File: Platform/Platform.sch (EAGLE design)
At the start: 30 parts, among them U1 LCD-16X2NOSILK, U2 LM2574N, X1 USBSMD, Y1 RESONATORSMD

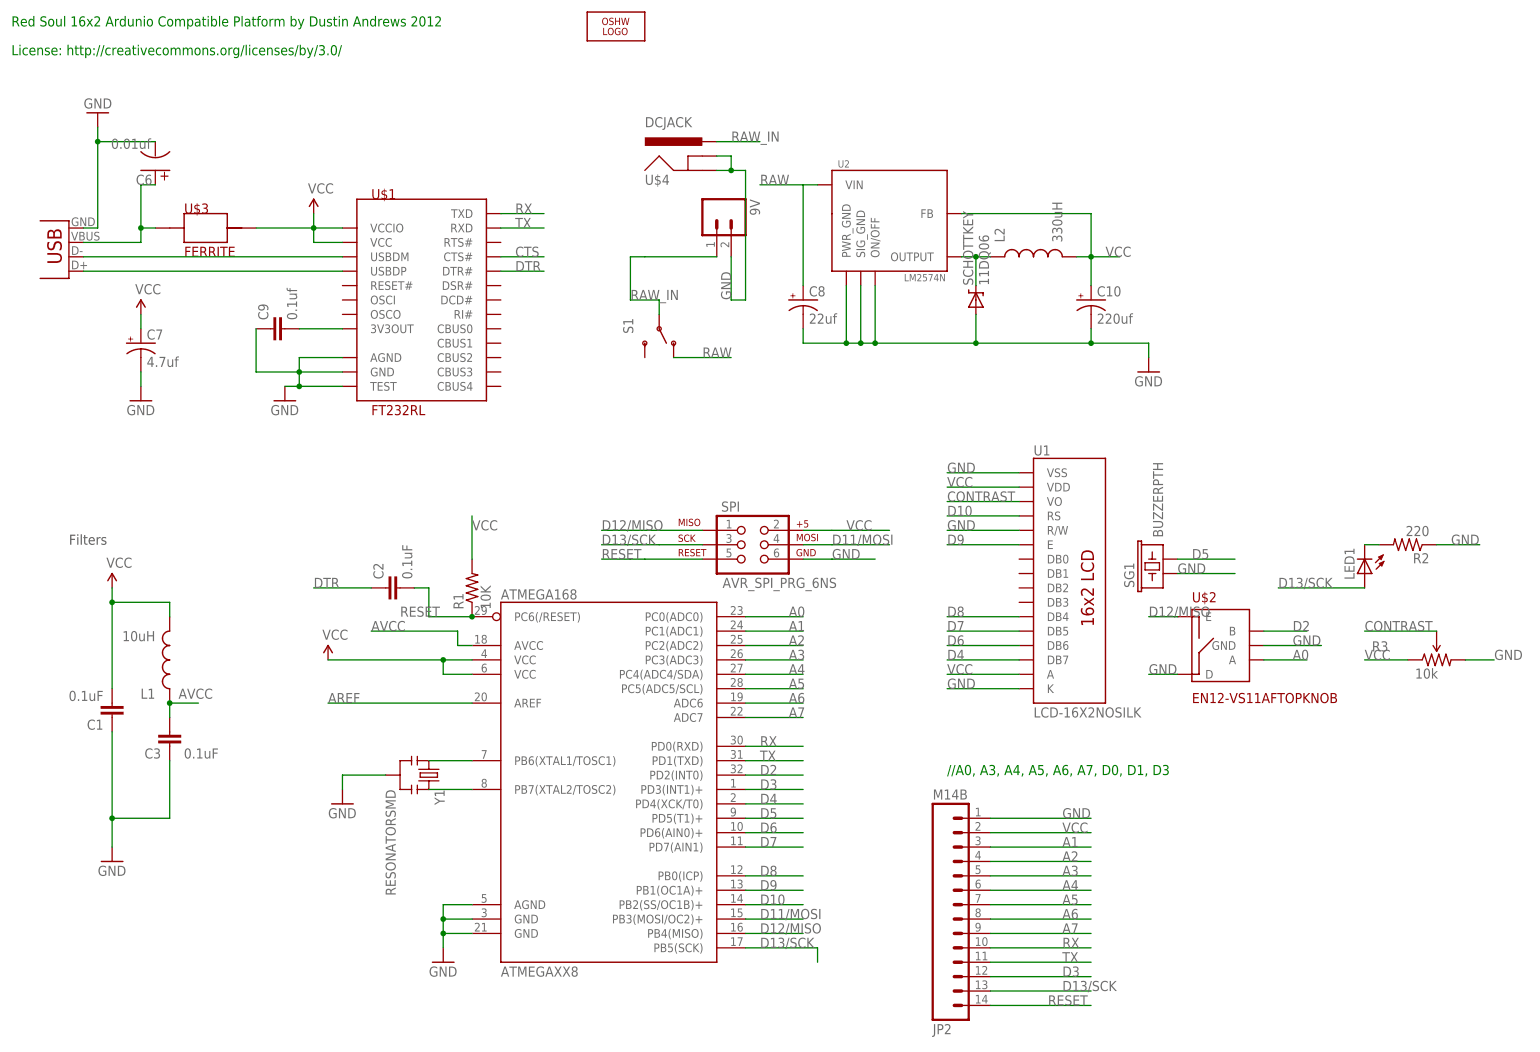
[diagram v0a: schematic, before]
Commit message: prototype 3
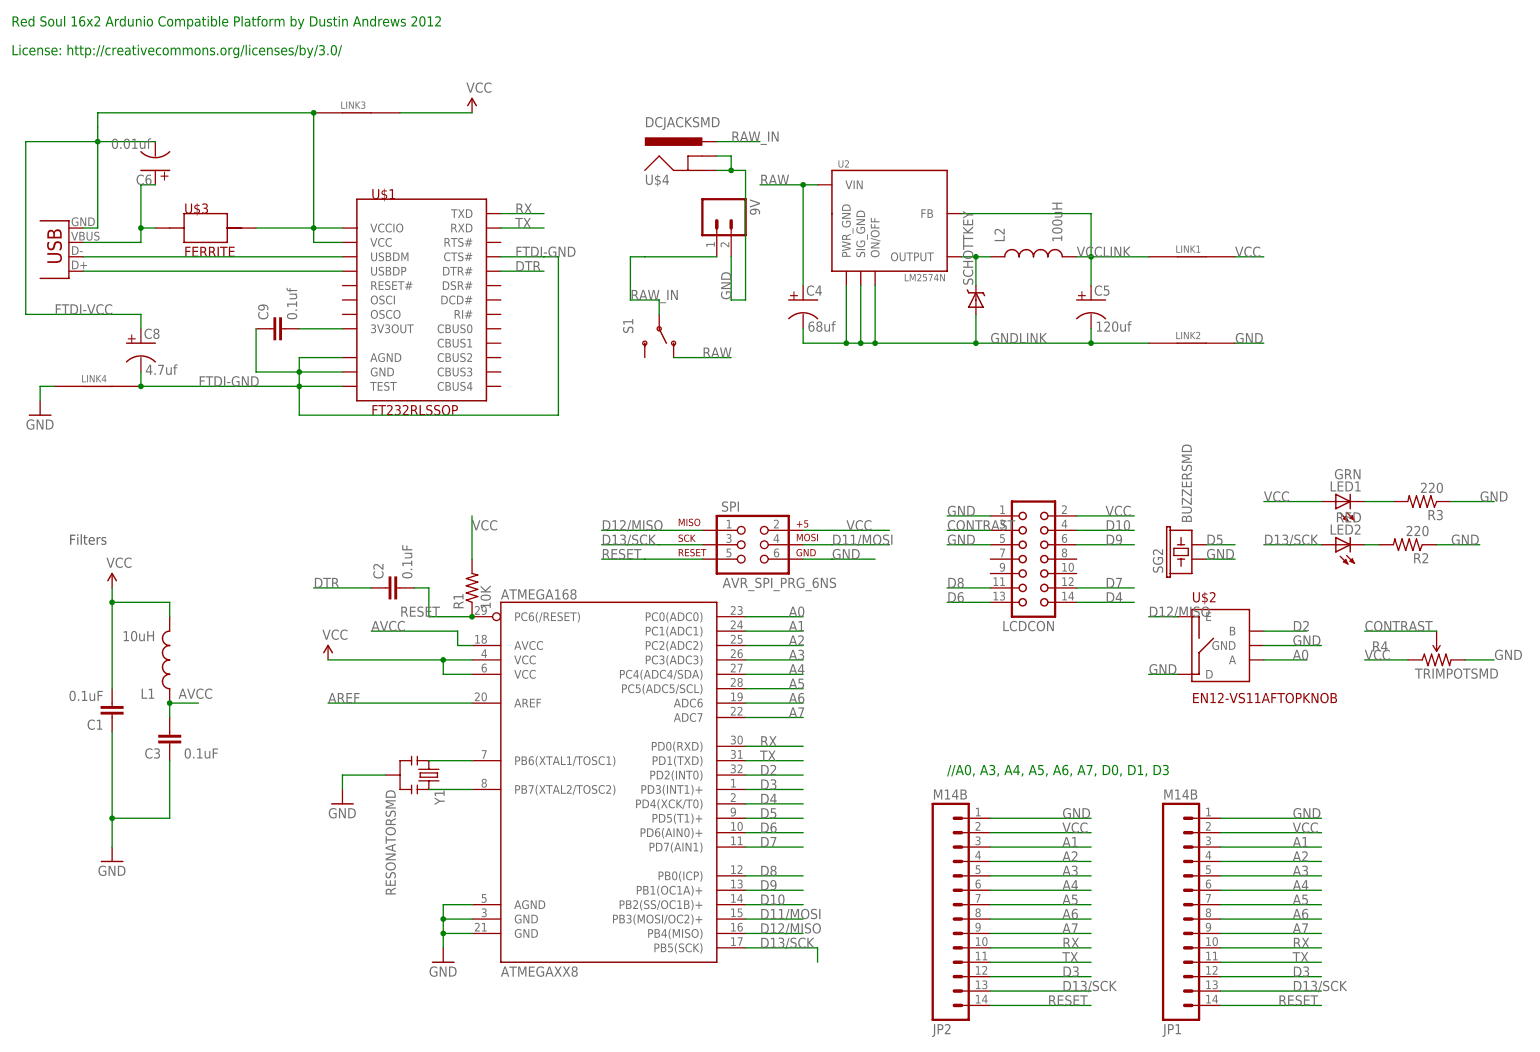
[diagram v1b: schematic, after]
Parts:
- removed C10: 220uf, SparkFun:CAP_POLPTH1
- removed C7: 4.7uf, SparkFun:CAP_POLPTH1
- removed LOGO1: OSHW_LOGO_10MIL, ohw-logo:OSHW_LOGO_10MIL
- removed SG1: BUZZERPTH, SparkFun:BUZZERPTH
- removed U1: LCD-16X2NOSILK, SparkFun:LCD-16X2NOSILK
- added C4: 68uf, Dustin:CAP_POLF80
- added C5: 120uf, Dustin:CAP_POL8X10
- added JP1: M14B, Dustin:M14B
- added LCDCON: (no value), con-harting:CON14
- added LED2: RED, SparkFun:LED1206
- added LINK1, LINK2, LINK3, LINK4: LINK, Dustin:LINK
- added R4: TRIMPOTSMD, SparkFun:TRIMPOTSMD
- added SG2: BUZZERSMD, SparkFun:BUZZERSMD
- C8: value 22uf -> 4.7uf; device SparkFun:CAP_POLPTH1 -> Dustin:CAP_POLCAP-B
- L2: value 330uH -> 100uH; device SparkFun:INDUCTOR1206H* -> SparkFun:INDUCTOR0805
- LED1: value (none) -> GRN; device SparkFun:LED3MM -> SparkFun:LED1206
- R3: value 10k -> 220; device SparkFun:TRIMPOTPTH -> SparkFun:RESISTOR0805-RES
- SCHOTTKEY: value 11DQ06 -> DIODE-SCHOTTKY; device SparkFun:DIODE-ZENERPTH -> Dustin:DIODE-SCHOTTKY
- U$1: value FT232RL -> FT232RLSSOP; device Dustin:FT232RL -> Dustin:FT232RLSSOP
- U$4: value DCJACK -> DCJACKSMD; device Dustin:DCJACK -> Dustin:DCJACKSMD
- U2: device Dustin:LM2574N -> Dustin:LM2574NSOIC8
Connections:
- removed net CTS: U$1.CTS#
- new net FTDI-GND: C8.-, C9.1, LINK4.P$2, U$1.AGND, U$1.CTS#, U$1.GND, U$1.TEST
- new net FTDI-VCC: C6.-, C8.+, LINK3.P$1, U$1.VCC, U$1.VCCIO, U$3.P$2, X1.GND
- new net GNDLINK: C4.-, C5.-, LINK2.P$1, SCHOTTKEY.A, U2.ON/OFF, U2.PWR_GND, U2.SIG_GND
- new net N$7: LED1.C, R3.2
- new net VCCLINK: C5.+, L2.2, LINK1.P$1, U2.FB
- net A1: now also JP1.3
- net A2: now also JP1.4
- net A3: now also JP1.5
- net A4: now also JP1.6
- net A5: now also JP1.7
- net A6: now also JP1.8
- net A7: now also JP1.9
- net CONTRAST: now also LCDCON.3, R4.WIPER; no longer R3.WIPER, U1.VO
- net D10: now also LCDCON.4; no longer U1.RS
- net D13/SCK: now also JP1.13, LED2.A; no longer LED1.A
- net D3: now also JP1.12
- net D4: now also LCDCON.14; no longer U1.DB7
- net D5: now also SG2.2; no longer SG1.2
- net D6: now also LCDCON.13; no longer U1.DB6
- net D7: now also LCDCON.12; no longer U1.DB5
- net D8: now also LCDCON.11; no longer U1.DB4
- net D9: now also LCDCON.6; no longer U1.E
- net GND: now also JP1.1, LCDCON.1, LCDCON.5, LINK2.P$2, LINK4.P$1, R3.1, R4.CW, SG2.1; no longer C10.-, C6.-, C7.-, C8.-, C9.1, R3.CW, SCHOTTKEY.A, SG1.1, U$1.AGND, U$1.GND, U$1.TEST, U1.K, U1.R/W, U1.VSS, U2.ON/OFF, U2.PWR_GND, U2.SIG_GND, X1.GND
- net N$2: now also LED2.C; no longer LED1.C
- net RAW: now also C4.+; no longer C8.+
- net RESET: now also JP1.14
- net RX: now also JP1.10
- net TX: now also JP1.11
- net VCC: now also JP1.2, LCDCON.2, LED1.A, LINK1.P$2, LINK3.P$2, R4.CCW; no longer C10.+, C7.+, L2.2, R3.CCW, U$1.VCC, U$1.VCCIO, U$3.P$2, U1.A, U1.VDD, U2.FB
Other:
- moved on the sheet: LED1
